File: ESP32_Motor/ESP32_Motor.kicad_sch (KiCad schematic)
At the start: 20 parts, among them J1 Conn_01x03, M1 Motor_DC, Q1 IRLML9301, Q2 Q_NPN_EBC, SW1 RotaryEncoder_Switch, U1 AMS1117-3.3, U2 YD-ESP32-S3

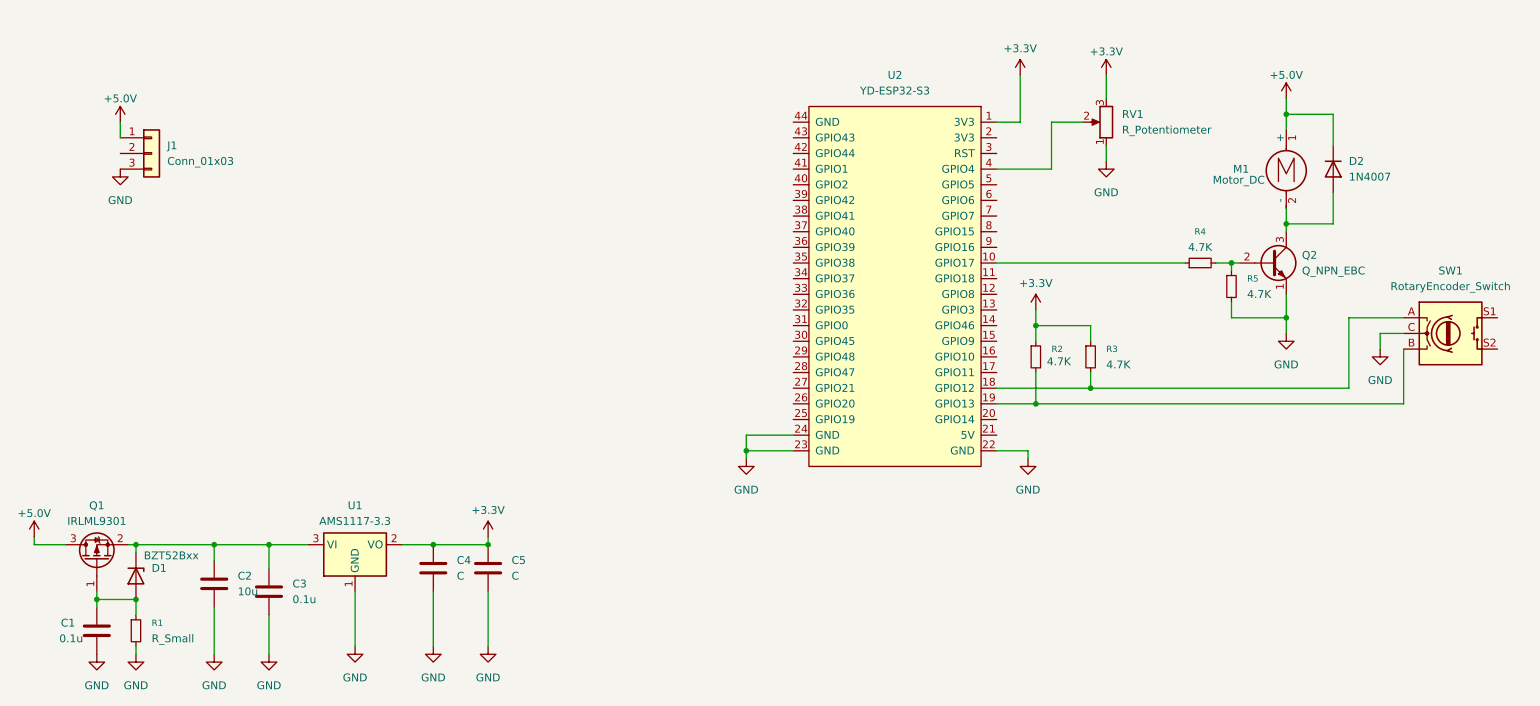
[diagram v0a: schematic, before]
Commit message: M_5_2_19_08_26
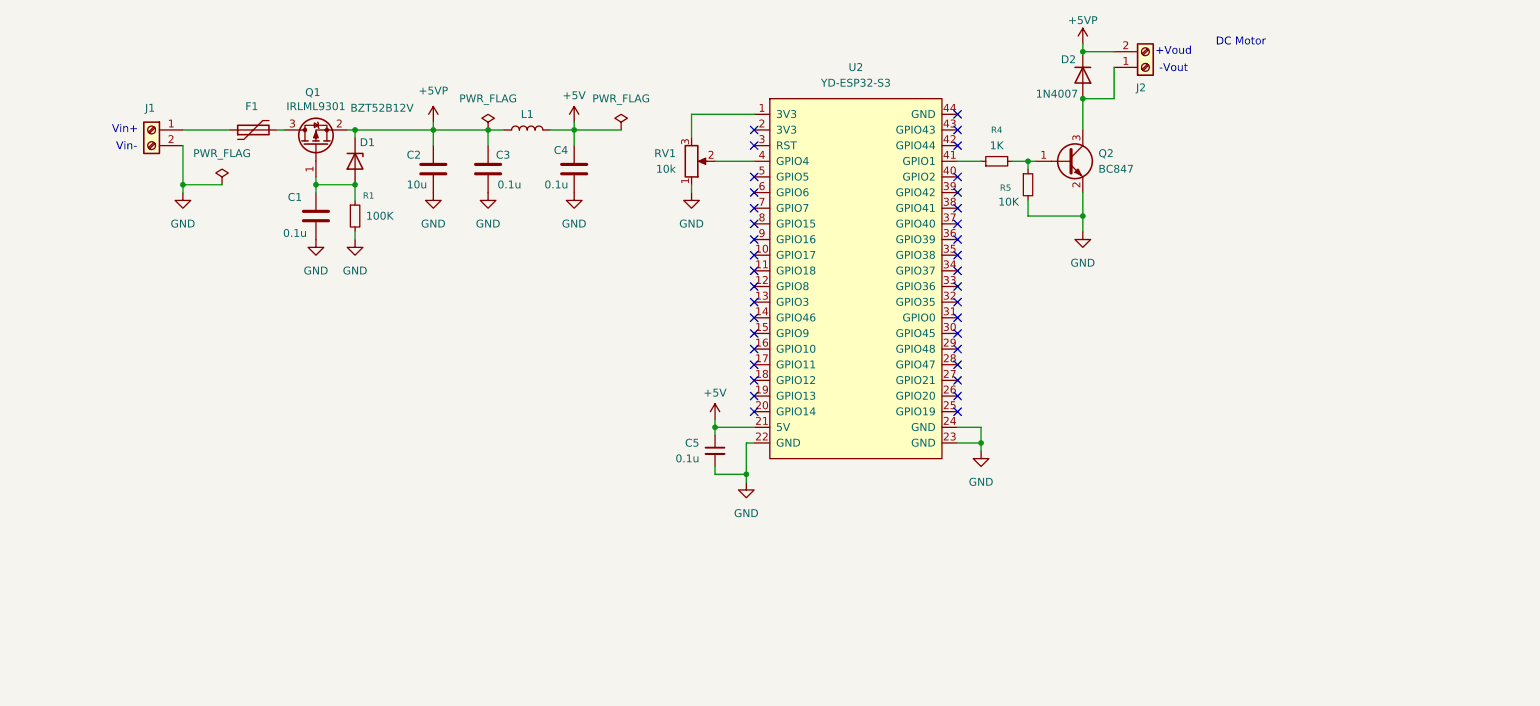
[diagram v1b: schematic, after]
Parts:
- removed C5: C, symbol Device:C
- removed J1: Conn_01x03, symbol Connector_Generic:Conn_01x03
- removed M1: Motor_DC, symbol Motor:Motor_DC
- removed Q2: Q_NPN_EBC, symbol Transistor_BJT:Q_NPN_EBC
- removed R2, R3: 4.7K, symbol Device:R_Small
- removed SW1: RotaryEncoder_Switch, symbol Device:RotaryEncoder_Switch
- removed U1: AMS1117-3.3, Package_TO_SOT_SMD:SOT-223-3_TabPin2, symbol Regulator_Linear:AMS1117-3.3
- added C5: 0.1u, Capacitor_SMD:C_0805_2012Metric, symbol Device:C_Small
- added F1: Polyfuse, Fuse:Fuse_Bourns_MF-SM_7.98x5.44mm, symbol Device:Polyfuse
- added J1, J2: Screw_Terminal_01x02, TerminalBlock_Phoenix:TerminalBlock_Phoenix_MKDS-1,5-2-5.08_1x02_P5.08mm_Horizontal, symbol Connector:Screw_Terminal_01x02
- added L1: L, Inductor_SMD:L_0805_2012Metric, symbol Device:L
- added Q2: BC847, Package_TO_SOT_SMD:SOT-23, symbol Transistor_BJT:BC847
- C1, C2, C3: footprint (none) -> Capacitor_SMD:C_0805_2012Metric
- C4: value C -> 0.1u; footprint (none) -> Capacitor_SMD:C_0805_2012Metric
- D1: value BZT52Bxx -> BZT52B12V
- R1: value R_Small -> 100K; footprint (none) -> Resistor_SMD:R_0805_2012Metric_Pad1.20x1.40mm_HandSolder
- R4: value 4.7K -> 1K; footprint (none) -> Resistor_SMD:R_0805_2012Metric_Pad1.20x1.40mm_HandSolder
- R5: value 4.7K -> 10K; footprint (none) -> Resistor_SMD:R_0805_2012Metric_Pad1.20x1.40mm_HandSolder
- RV1: value R_Potentiometer -> 10k; footprint (none) -> Potentiometer_SMD:Potentiometer_ACP_CA14-VSMD_Vertical
- U2: footprint Shared:YD-ESP32-S3 -> YD-ESP32-S3-main:YD-ESP32-S3
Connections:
- net GND: now also C5.2, J1.2 (Pin_2), Q2.2 (E)
- net at R4.2, R5.1: now also Q2.1 (B)
- net at D2.2 (A): now also J2.1 (Pin_1), Q2.3 (C)
- net +5VP: now reaches C2.1, C3.1, D1.1 (K), Q1.2 (S)
- net +5VP: now also D2.1 (K), J2.2 (Pin_2), L1.1
- net at U2.10 (GPIO17): no longer R4.1
- net +5V: now reaches U2.21 (5V)
- net +5V: now also C4.1, C5.1, L1.2
- net at U2.41 (GPIO1): now also R4.1
- net +3.3V: no longer names the net of RV1.3, U2.1 (3V3)
- net +3.3V: no longer C4.1
- net +5.0V: no longer names the net of Q1.3 (D)
- net +5.0V: now also F1.2; no longer D2.1 (K)
- new net: F1.1, J1.1 (Pin_1)
- no-connect marks 0 -> 37
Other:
- note added: "+Voud"
- note added: "-Vout"
- note added: "DC Motor"
- note added: "Vin+"
- note added: "Vin-"
- moved on the sheet: C1, C2, C3, C4, D1, D2, Q1, R1, R4, R5, RV1, U2
